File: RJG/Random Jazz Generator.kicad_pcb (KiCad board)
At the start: 2 copper layers, 109 parts, among them J101 EuroPower, J102 CV, J103 RND, J104 Gate, J105 Trig1, J106 Trig2, J107 Clock, J108 Trig3, J109 Trig4, Q101 BC557, Q102 BC547, Q201 BC547, Q202 BC547, Q401 BC547, Q402 BC547, SW101 Reset, SW301 Reload, SW401 Duration Length, SW402 Reload, U101 L7805, U102 4520, U103 TL082, U201 74LS04, U202 74LS595, U301 74HCT4051, U302 74HCT40105, U303 74LS157, U304 74LS157, U401 4520, U402 74LS74, U403 74LS85, U404 74LS157, U405 SST39SF010, U407 74LS173

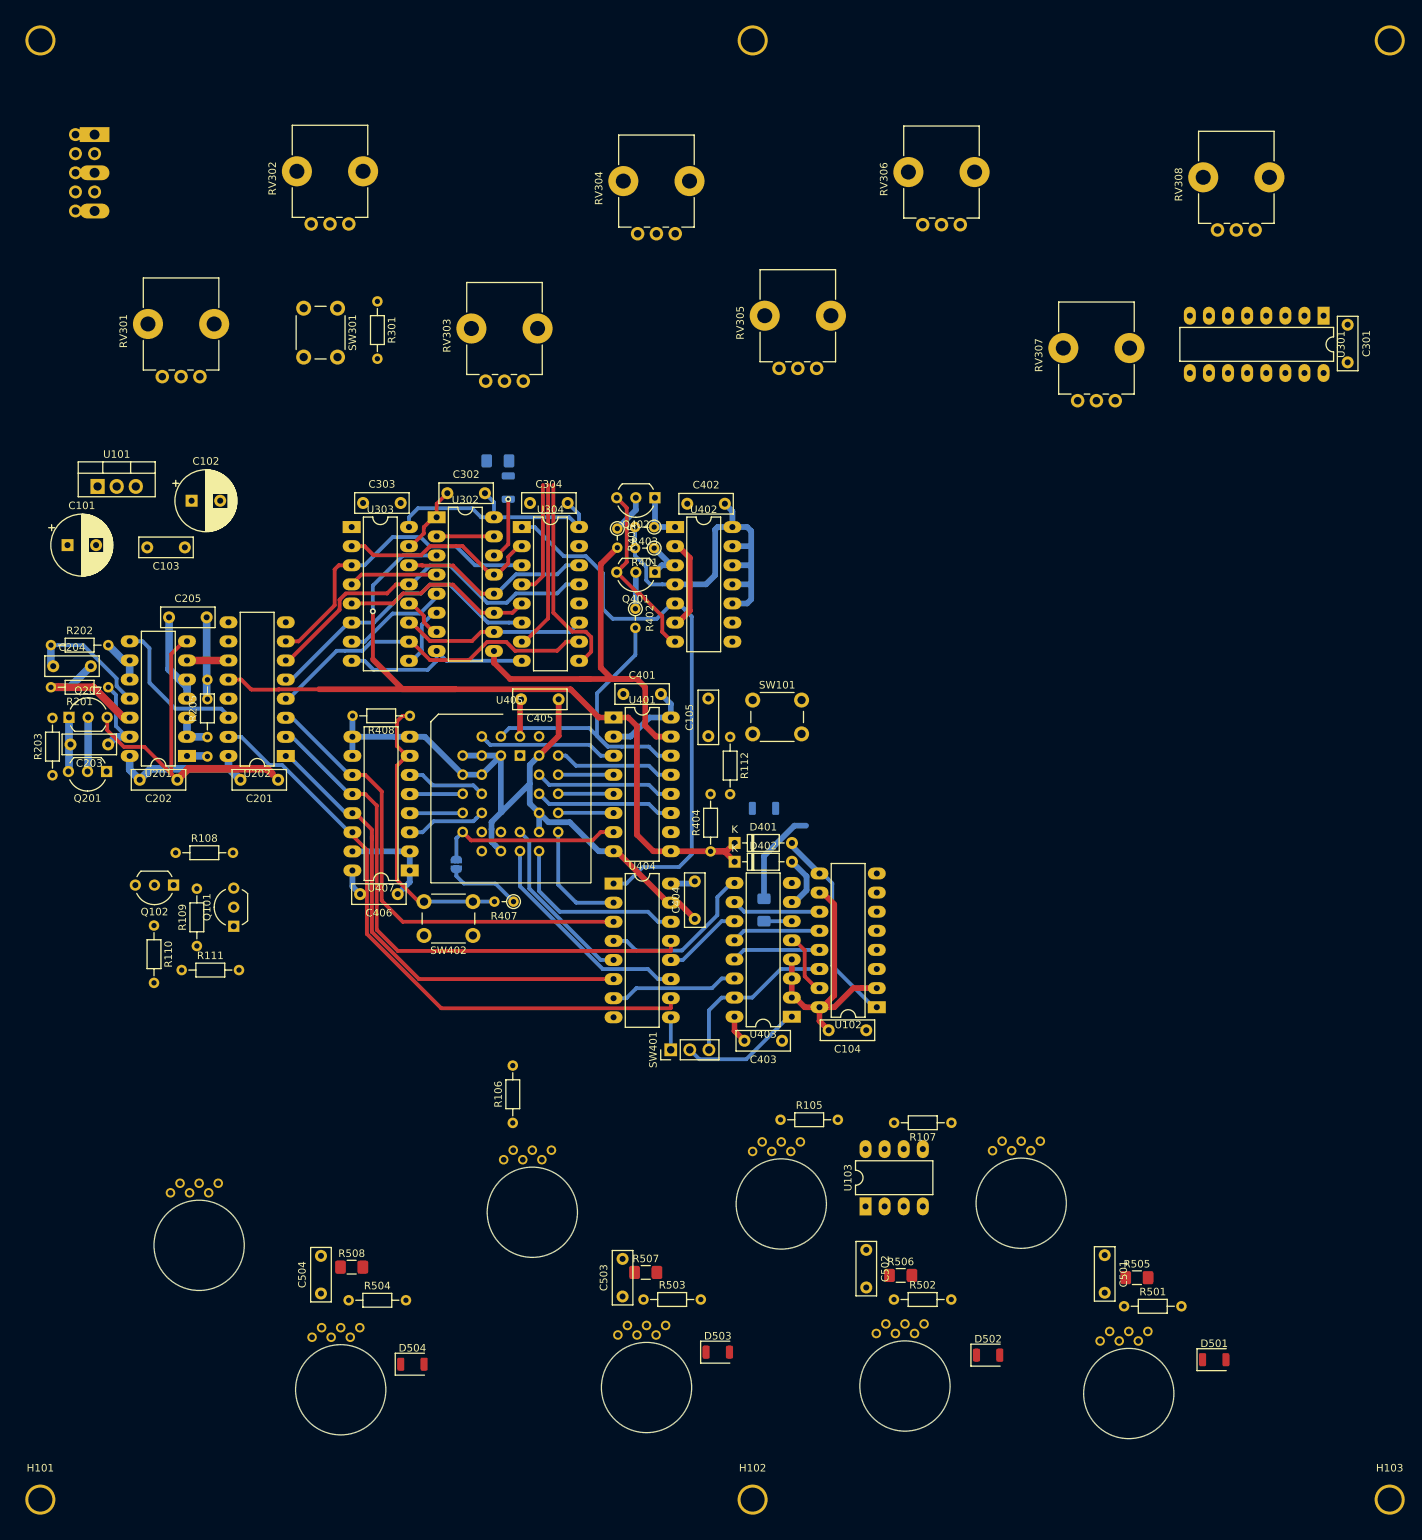
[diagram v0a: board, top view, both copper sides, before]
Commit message: Finsihed layout
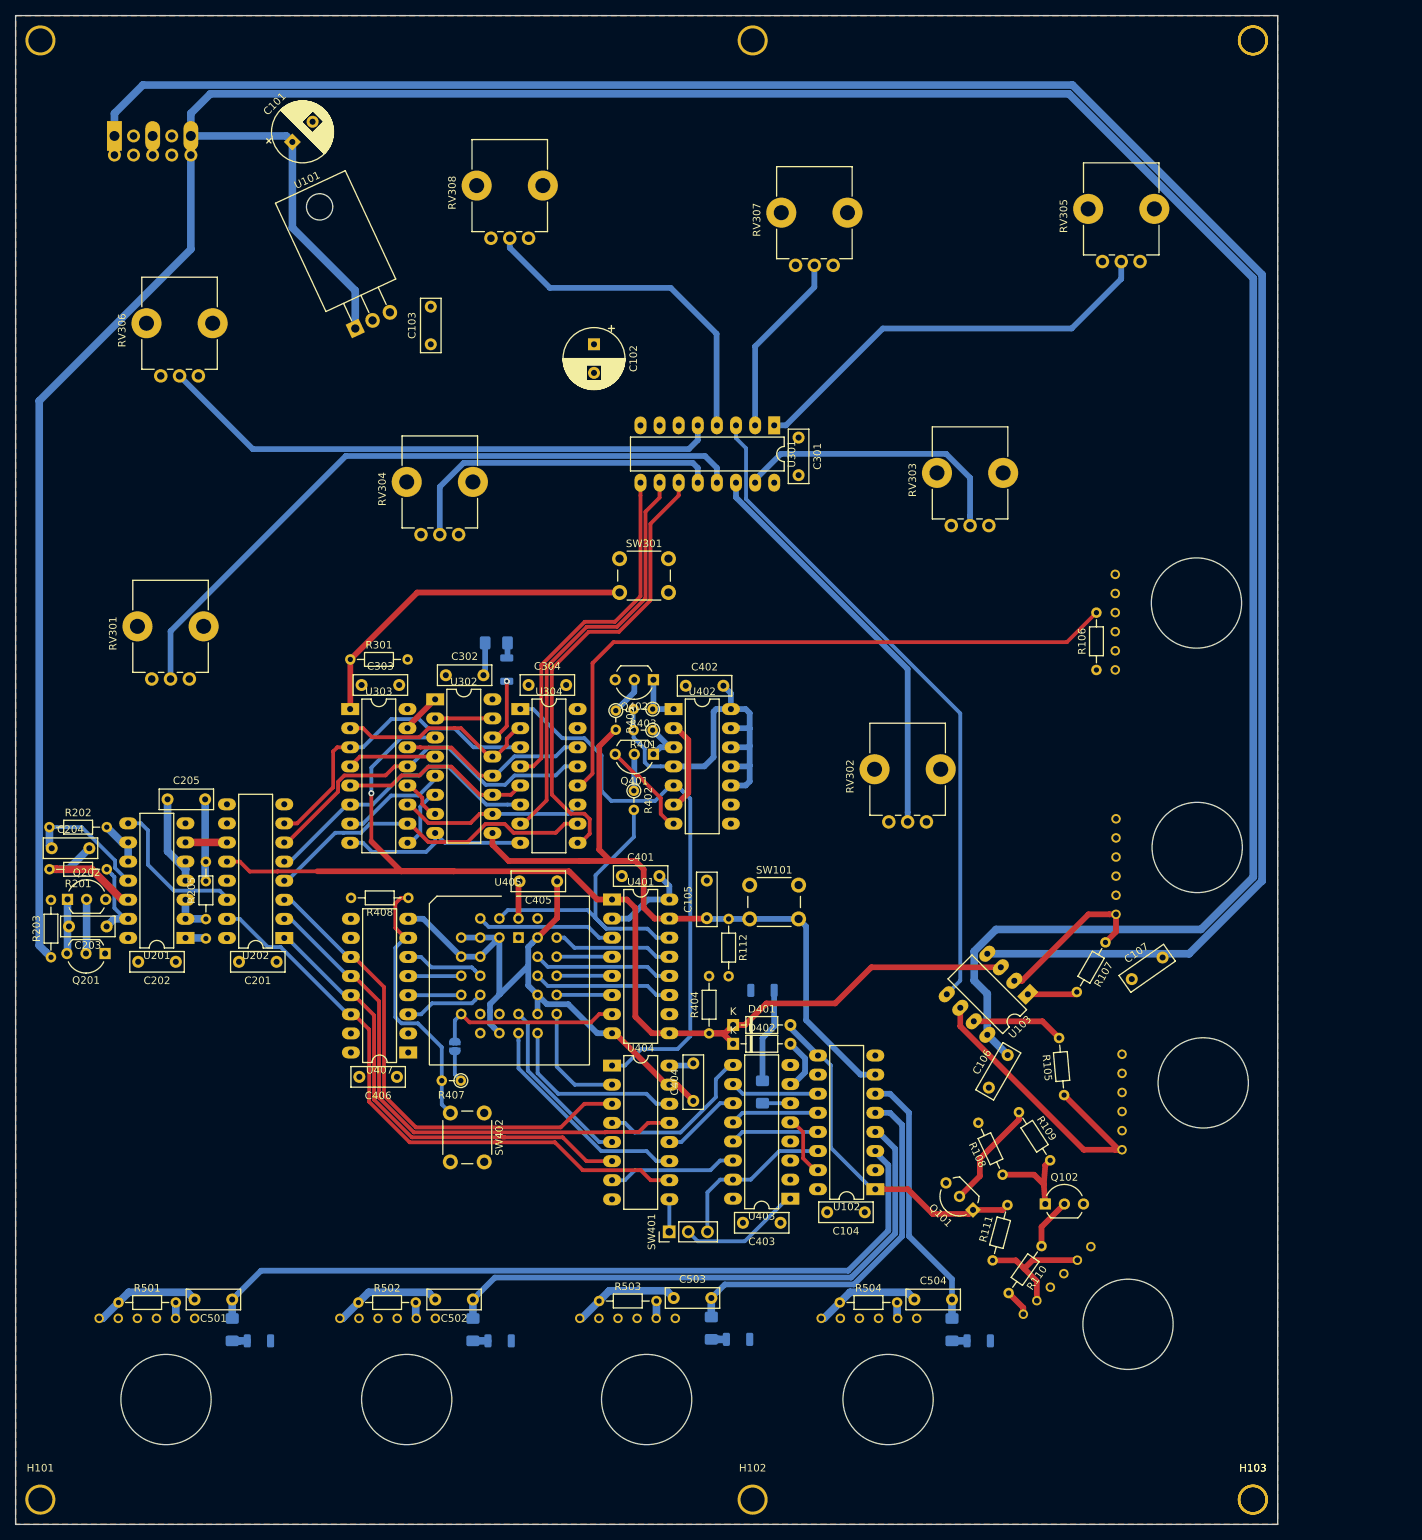
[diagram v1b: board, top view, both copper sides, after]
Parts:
- removed the H103 at (194.7, 209.3)
- added C106: 100n, Capacitor_THT:C_Disc_D7.0mm_W2.5mm_P5.00mm, F.Cu at (141.4, 154.5)
- added C107: 100n, Capacitor_THT:C_Disc_D7.0mm_W2.5mm_P5.00mm, F.Cu at (160.4, 140.1)
- added H103 (x2): Mounting_Holes, Kosmo_panel:Kosmo_Panel_Dual_Mounting_Holes, F.Cu at (176.5, 209.3)
- D501, D502, D503, D504, R505, R506, R507, R508: moved to B.Cu
- U101: footprint Package_TO_SOT_THT:TO-220-3_Vertical -> Package_TO_SOT_THT:TO-220-3_Horizontal_TabDown
- moved R501 133.7 mm to (25.7, 183.1)
- moved J105 128.0 mm to (32.0, 196.0)
- moved D501 127.0 mm to (44.4, 188.2), turned to 180 degrees
- moved R110 125.5 mm to (148.4, 175.6), turned to 235 degrees
- moved J107 123.9 mm to (159.9, 186.0), turned to 225 degrees
- moved Q102 123.4 mm to (148.9, 170.0), turned to 0 degrees
- moved R505 120.5 mm to (40.8, 186.7), turned to 270 degrees
- moved J103 119.8 mm to (169.0, 90.1), turned to 270 degrees
- moved R108 118.0 mm to (143.2, 166.1), turned to 115 degrees
- moved C501 116.1 mm to (40.8, 182.7), turned to 180 degrees
- moved R111 114.5 mm to (141.9, 177.5), turned to 75 degrees
- moved R109 111.5 mm to (145.4, 157.8), turned to 303 degrees
- moved RV302 110.5 mm to (133.1, 119.2)
- moved Q101 105.3 mm to (139.3, 170.8), turned to 135 degrees
- moved RV306 103.3 mm to (36.3, 59.9)
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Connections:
- U103 pad 1: Net-(R105-Pad2) -> Net-(R107-Pad2)
- U103 pad 2: Net-(J102-PadT) -> Net-(J104-PadT)
- U103 pad 3: /Notes/CV -> /Notes/Clk
- U103 pad 5: /Notes/Clk -> /Notes/CV
- U103 pad 6: Net-(J104-PadT) -> Net-(J102-PadT)
- U103 pad 7: Net-(R107-Pad2) -> Net-(R105-Pad2)
- U304 pad 4: Net-(U301-Pad11) -> Net-(U301-Pad9)
- U304 pad 9: Net-(U301-Pad9) -> Net-(U301-Pad11)
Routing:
- net +12V: track 0.00 -> 454.8 mm
- net -12V: track 0.00 -> 291.3 mm
- net Net-(C501-Pad1): track 0.00 -> 104.8 mm
- net +5V: track 173.5 -> 76.8 mm
- net /Notes/CV1: track 0.00 -> 91.3 mm
- net /Notes/CV: track 0.00 -> 88.7 mm
- net /Notes/RND: track 0.00 -> 87.1 mm
- net Net-(C502-Pad1): track 0.00 -> 77.1 mm
- net /Notes/CV6: track 0.00 -> 75.4 mm
- net GND: track 218.6 -> 155.2 mm
- net /Notes/CV5: track 0.00 -> 56.5 mm
- net /Notes/CV2: track 0.00 -> 54.6 mm
- net Net-(C503-Pad2): track 0.00 -> 50.3 mm
- net /Notes/Reload: track 0.00 -> 46.1 mm
- net Net-(U301-Pad11): track 15.4 -> 61.2 mm
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- added copper zone on F.Cu, net +5V
- added copper zone on B.Cu, net GND
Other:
- board outline added: 167.8 x 200.6 mm
